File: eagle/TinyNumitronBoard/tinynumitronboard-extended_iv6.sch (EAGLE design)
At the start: 36 parts

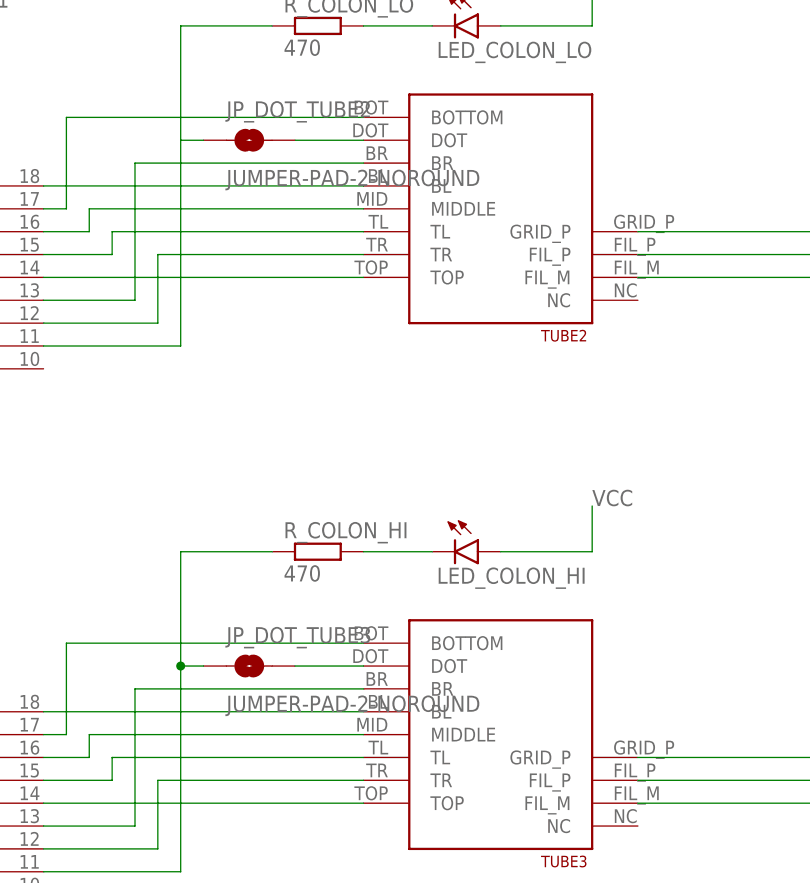
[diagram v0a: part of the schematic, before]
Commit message: Still optimizing/reviewing
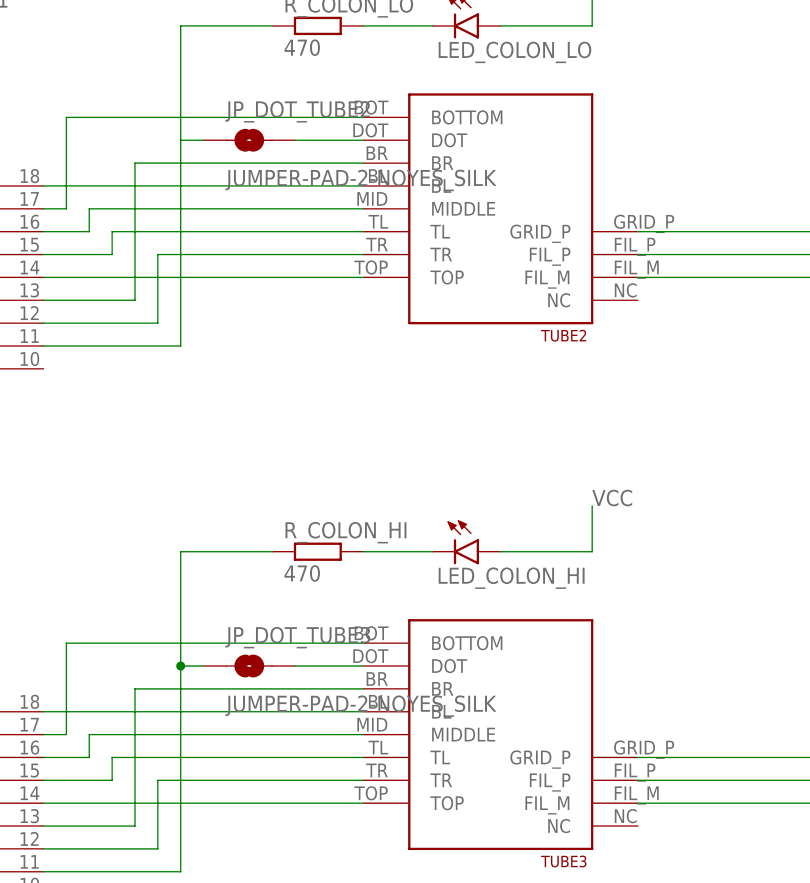
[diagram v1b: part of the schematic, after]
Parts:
- JP_DOT_TUBE2, JP_DOT_TUBE3: value JUMPER-PAD-2-NOROUND -> JUMPER-PAD-2-NOYES_SILK; device SparkFun-Passives:JUMPER-PAD-2-NOROUND -> SparkFun-Passives:JUMPER-PAD-2-NOYES_SILK
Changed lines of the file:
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@@
 <part name="LED_COLON_LO" library="SparkFun-LED" deviceset="LED" device="1206"/>
 <part name="R_COLON_LO" library="resistor" deviceset="R-EU_" device="M1206" value="470"/>
-<part name="JP_DOT_TUBE2" library="SparkFun-Passives" deviceset="JUMPER-PAD-2-NO" device="ROUND"/>
+<part name="JP_DOT_TUBE2" library="SparkFun-Passives" deviceset="JUMPER-PAD-2-NO" device="YES_SILK" value="JUMPER-PAD-2-NOYES_SILK"/>
 <part name="LED_COLON_HI" library="SparkFun-LED" deviceset="LED" device="1206"/>
 <part name="R_COLON_HI" library="resistor" deviceset="R-EU_" device="M1206" value="470"/>
-<part name="JP_DOT_TUBE3" library="SparkFun-Passives" deviceset="JUMPER-PAD-2-NO" device="ROUND"/>
+<part name="JP_DOT_TUBE3" library="SparkFun-Passives" deviceset="JUMPER-PAD-2-NO" device="YES_SILK" value="JUMPER-PAD-2-NOYES_SILK"/>
 <part name="TP1" library="testpad" deviceset="TP" device="B2,54" value="TPB2,54"/>
 </parts>
